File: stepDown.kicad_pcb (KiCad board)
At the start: 2 copper layers, 48 parts, among them P1 ScrewIN, P2 PowerPoleOUT, P3 PowerPoleIN, P4 ScrewOUT, Q1 M1, Q2 M2, Q3 M3, Q4 M4, U1 LM25119

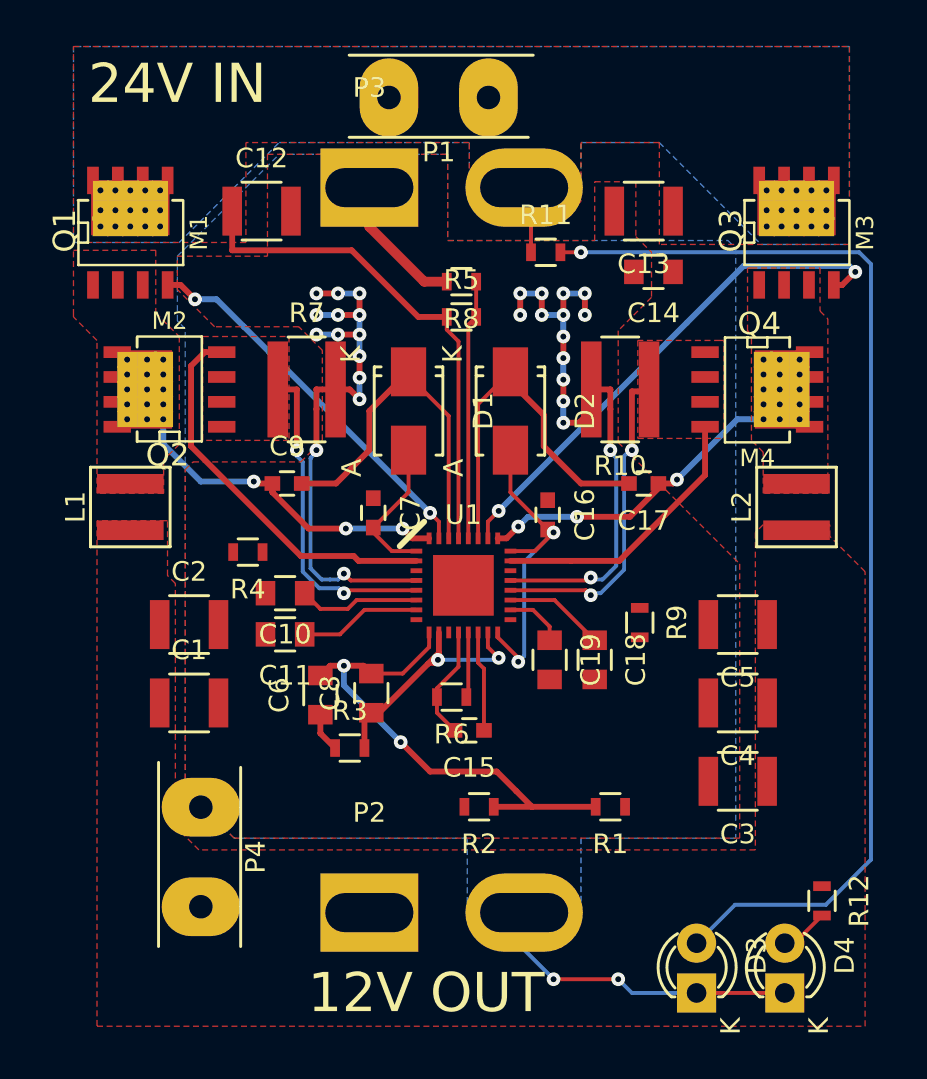
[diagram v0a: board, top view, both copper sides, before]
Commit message: weiter gemacht...
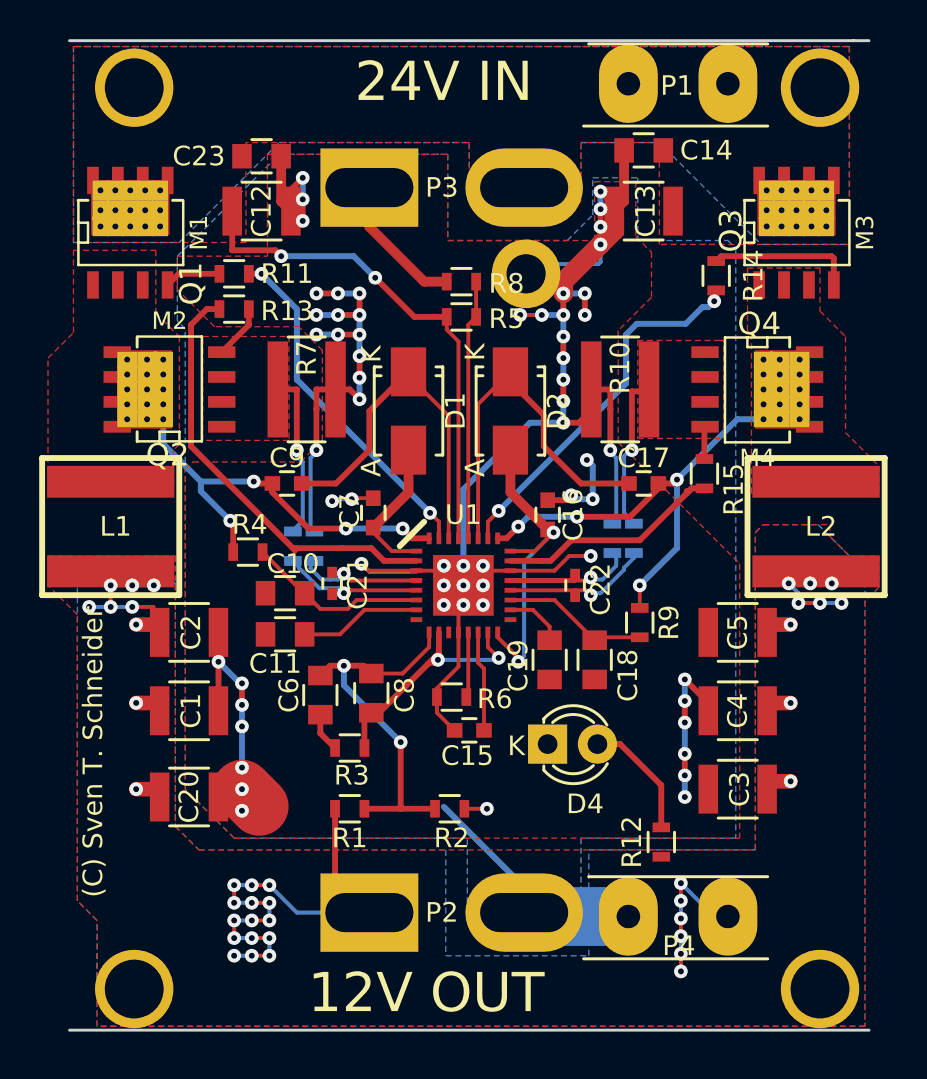
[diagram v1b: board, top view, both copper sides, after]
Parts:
- removed D3: LED, LEDs:LED-3MM
- added C20: Cout, Capacitors_SMD:C_1210, F.Cu at (54.0, 106.8)
- added C21: 300p, Capacitors_SMD:C_0402, F.Cu at (61.3, 95.9)
- added C22: 300p, Capacitors_SMD:C_0402, F.Cu at (73.7, 96.0)
- added C23: Cinx, Capacitors_SMD:C_0805, F.Cu at (57.7, 74.1)
- added R13: 4,7, Resistors_SMD:R_0603, F.Cu at (56.3, 81.9)
- added R14: 4,7, Resistors_SMD:R_0603, F.Cu at (80.9, 80.2)
- added R15: 4,7, Resistors_SMD:R_0603, F.Cu at (80.3, 90.3)
- added R16: 10, Resistors_SMD:R_0603, B.Cu at (59.3, 94.0)
- added R17: 10, Resistors_SMD:R_0603, B.Cu at (60.4, 94.0)
- added R18: 10, Resistors_SMD:R_0603, B.Cu at (76.7, 93.6)
- added R19: 10, Resistors_SMD:R_0603, B.Cu at (75.6, 93.6)
- added REF**: Pin_Header_Straight_1x01, Pin_Headers:Pin_Header_Straight_1x01, F.Cu at (86.2, 70.6)
- L1, L2: footprint Sven:Z_Coilcraft_XFL4020 -> Sven:Z_Coilcraft_XAL7070
- R11: value Rled1 -> 4,7
- moved P4 26.9 mm to (81.5, 112.9), turned to 180 degrees
- moved D4 17.5 mm to (72.3, 104.1), turned to 0 degrees
- moved P1 17.3 mm to (81.5, 70.4), turned to 180 degrees
- moved R11 15.9 mm to (56.3, 80.1)
- moved R1 13.3 mm to (62.2, 107.4), turned to 0 degrees
- moved R12 8.73 mm to (78.1, 109.1), turned to 90 degrees
- moved C14 6.22 mm to (77.2, 73.8)
- moved R2 1.50 mm to (67.3, 107.4), turned to 0 degrees
- moved L1 1.41 mm to (50.0, 93.0), turned to 270 degrees
- moved L2 1.41 mm to (86.0, 93.0), turned to 270 degrees
- moved C1 0.40 mm to (54.0, 102.4)
- moved C2 0.40 mm to (54.0, 98.4)
- moved C3 0.40 mm to (82.0, 106.4)
- moved C4 0.40 mm to (82.0, 102.4)
- moved C5 0.40 mm to (82.0, 98.4)
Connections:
- NT1 pad 1: /CSG1 -> Net-(NT1-Pad1)
- NT2 pad 1: /CSG2 -> Net-(NT2-Pad1)
- P1 pad 1: GND -> +24V
- Q1 pad G: /HO1 -> Net-(Q1-PadG)
- Q2 pad G: /LO1 -> Net-(Q2-PadG)
- Q2 pad S: /CS1 -> Net-(Q2-PadS)
- Q3 pad G: /HO2 -> Net-(Q3-PadG)
- Q4 pad G: /LO2 -> Net-(Q4-PadG)
- Q4 pad S: /CS2 -> Net-(Q4-PadS)
- R10 pad 1: /CS2 -> Net-(Q4-PadS)
- R11 pad 1: +24V -> Net-(Q1-PadG)
- R11 pad 2: Net-(D3-Pad2) -> /HO1
- R7 pad 1: /CS1 -> Net-(Q2-PadS)
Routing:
- net GND: track 60.4 -> 152.2 mm, vias 27 -> 60
- net Net-(D3-Pad2): track 57.2 -> 0.00 mm, vias 1 -> 0
- net +12V: track 0.00 -> 54.2 mm, vias 0 -> 39
- net /CS1: track 16.7 -> 7.70 mm, vias 2 -> 1
- net /CS2: track 16.7 -> 7.80 mm, vias 2 -> 1
- net Net-(Q2-PadS): track 0.00 -> 8.56 mm, vias 0 -> 1
- net Net-(Q4-PadS): track 0.00 -> 8.10 mm, vias 0 -> 1
- net Net-(Q3-PadG): track 0.00 -> 7.51 mm
- net /HO2: track 26.5 -> 19.1 mm
- net /SW2: track 16.2 -> 23.6 mm, vias 3 -> 4
- net /CSG1: track 14.2 -> 6.99 mm, vias 2 -> 1
- net Net-(NT1-Pad1): track 0.00 -> 6.46 mm, vias 0 -> 1
- net /FB: track 25.7 -> 19.7 mm
- net Net-(NT2-Pad1): track 0.00 -> 6.06 mm, vias 0 -> 1
- net /SW1: track 17.1 -> 21.4 mm, vias 3 -> 4
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- added copper zone on B.Cu, net +12V
- added copper zone on F.Cu, net Net-(Q2-PadS)
- added copper zone on F.Cu, net Net-(Q4-PadS)
- removed copper zone on F.Cu, net /CS1
- removed copper zone on F.Cu, net /CS2
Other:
- board outline added: 40.8 x 50.5 mm
- board text added: "(C) Sven T. Schneider"
